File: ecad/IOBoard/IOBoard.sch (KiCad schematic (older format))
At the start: 11 parts, among them J1 SN37A12B, J2 PJ-102A, J3 toEffectsBoard, J4 SN37A12A, U1 FS57003PLT2B2M2QE

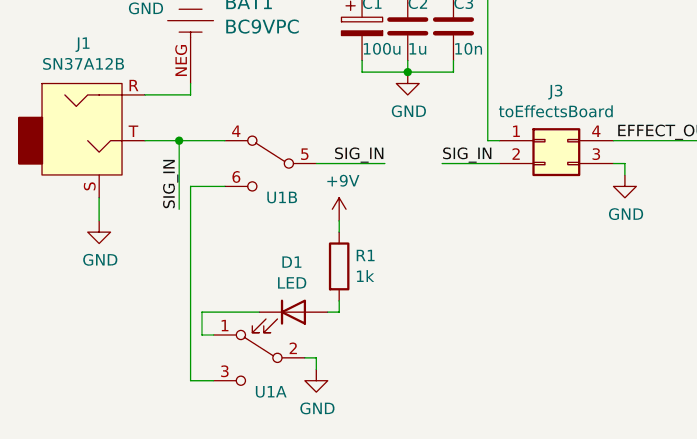
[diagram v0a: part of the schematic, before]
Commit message: Add LED datasheet
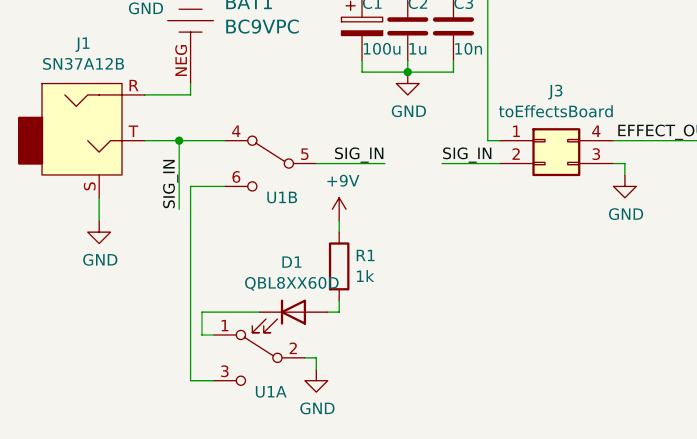
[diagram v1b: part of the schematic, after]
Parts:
- D1: value LED -> QBL8XX60D
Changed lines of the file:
@@
 P 1750 2500
 F 0 "D1" H 1743 2717 50  0000 C CNN
-F 1 "LED" H 1743 2626 50  0000 C CNN
+F 1 "QBL8XX60D" H 1743 2626 50  0000 C CNN
 F 2 "Diode_THT:D_DO-201AD_P3.81mm_Vertical_AnodeUp" H 1750 2500 50  0001 C CNN
-F 3 "~" H 1750 2500 50  0001 C CNN
+F 3 "http://www.qt-brightek.com/datasheet/QBL8XX60D.pdf" H 1750 2500 50  0001 C CNN
 F 4 "D" H 1750 2500 50  0001 C CNN "Spice_Primitive"
 F 5 "LED" H 1750 2500 50  0001 C CNN "Spice_Model"
